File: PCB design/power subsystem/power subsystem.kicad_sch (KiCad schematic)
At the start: 13 parts, among them Q1 IRLZ44N, U1 BQ27441-G1, U2 AMS1117-1.8

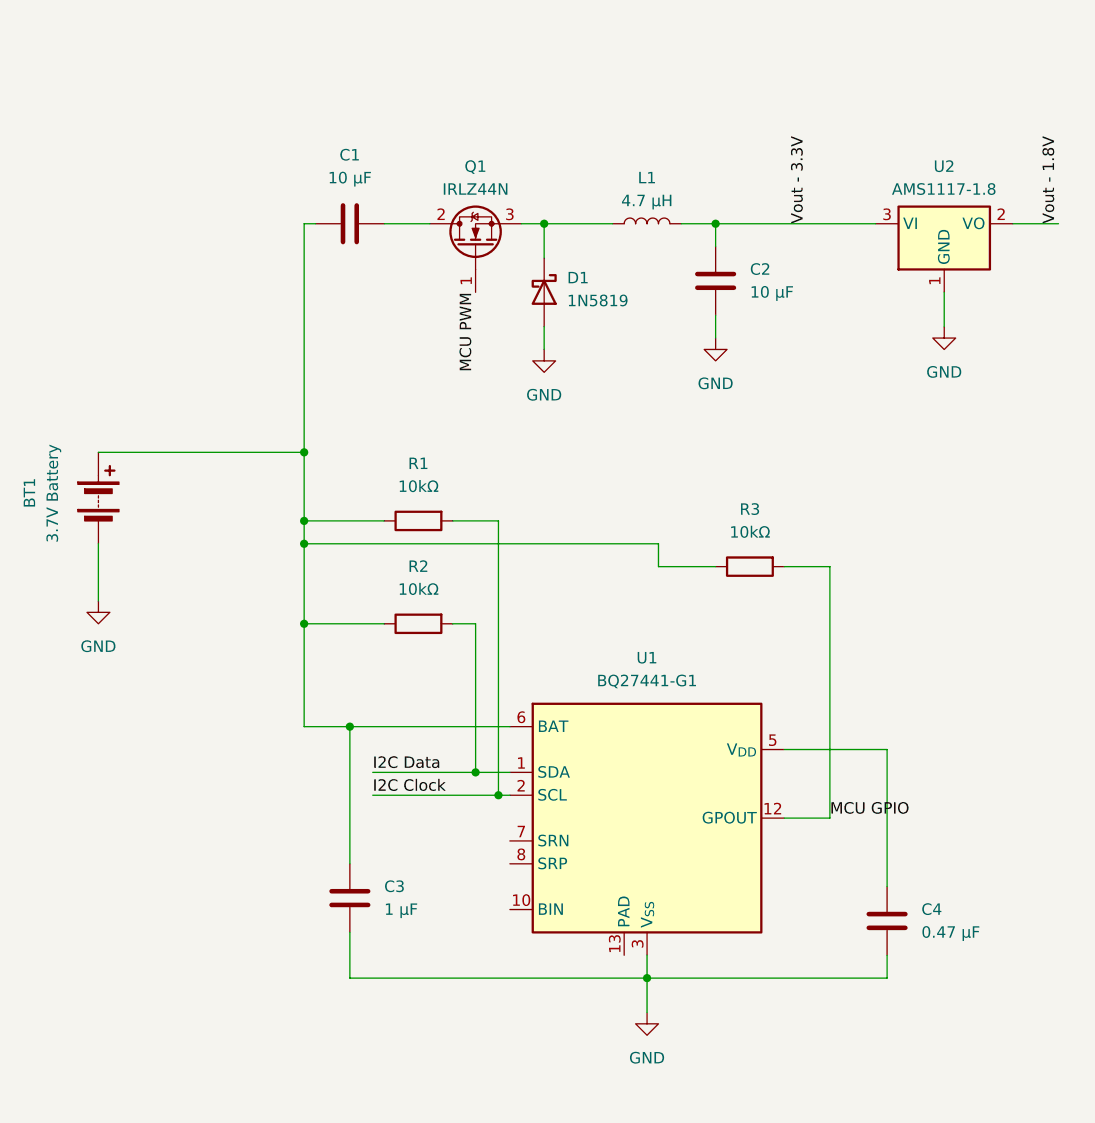
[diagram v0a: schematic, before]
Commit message: updated Notebook and pcb design files
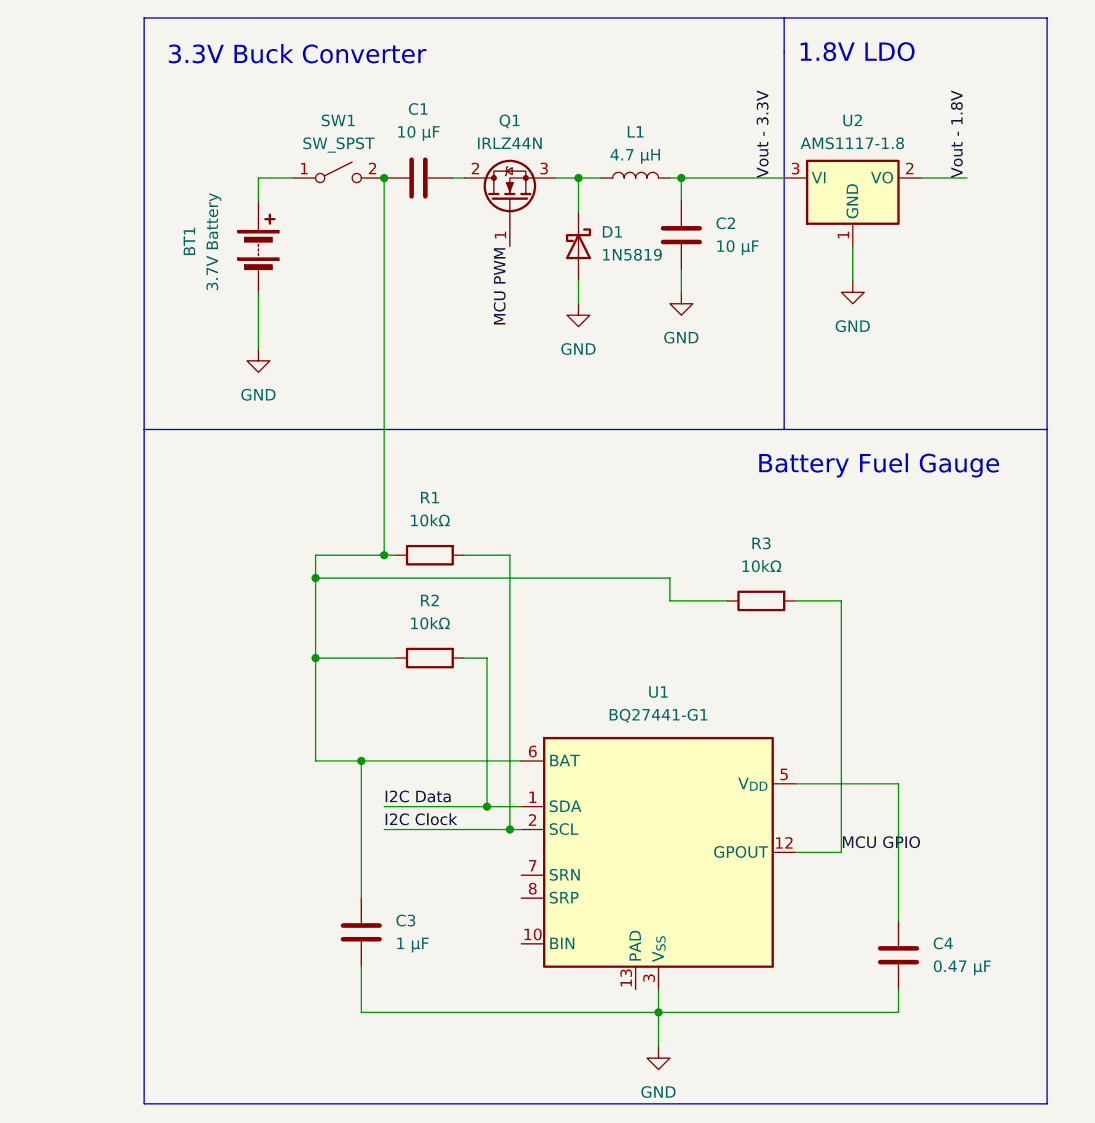
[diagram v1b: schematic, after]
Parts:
- added SW1: SW_SPST, symbol Switch:SW_SPST
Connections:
- net at C1.2, C3.1, R1.1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: now also SW1.2 (B); no longer BT1.1 (+)
- new net: BT1.1 (+), SW1.1 (A)
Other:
- note added: "1.8V LDO"
- note added: "3.3V Buck Converter"
- note added: "Battery Fuel Gauge"
- moved on the sheet: BT1, C1, C2, C3, C4, D1, L1, Q1, R1, R2, R3, U1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
